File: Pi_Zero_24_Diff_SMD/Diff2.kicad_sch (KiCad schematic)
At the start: 14 parts, among them J7 Diff Out, J8 Diff Out, U7 AM26C31, U8 AM26C31

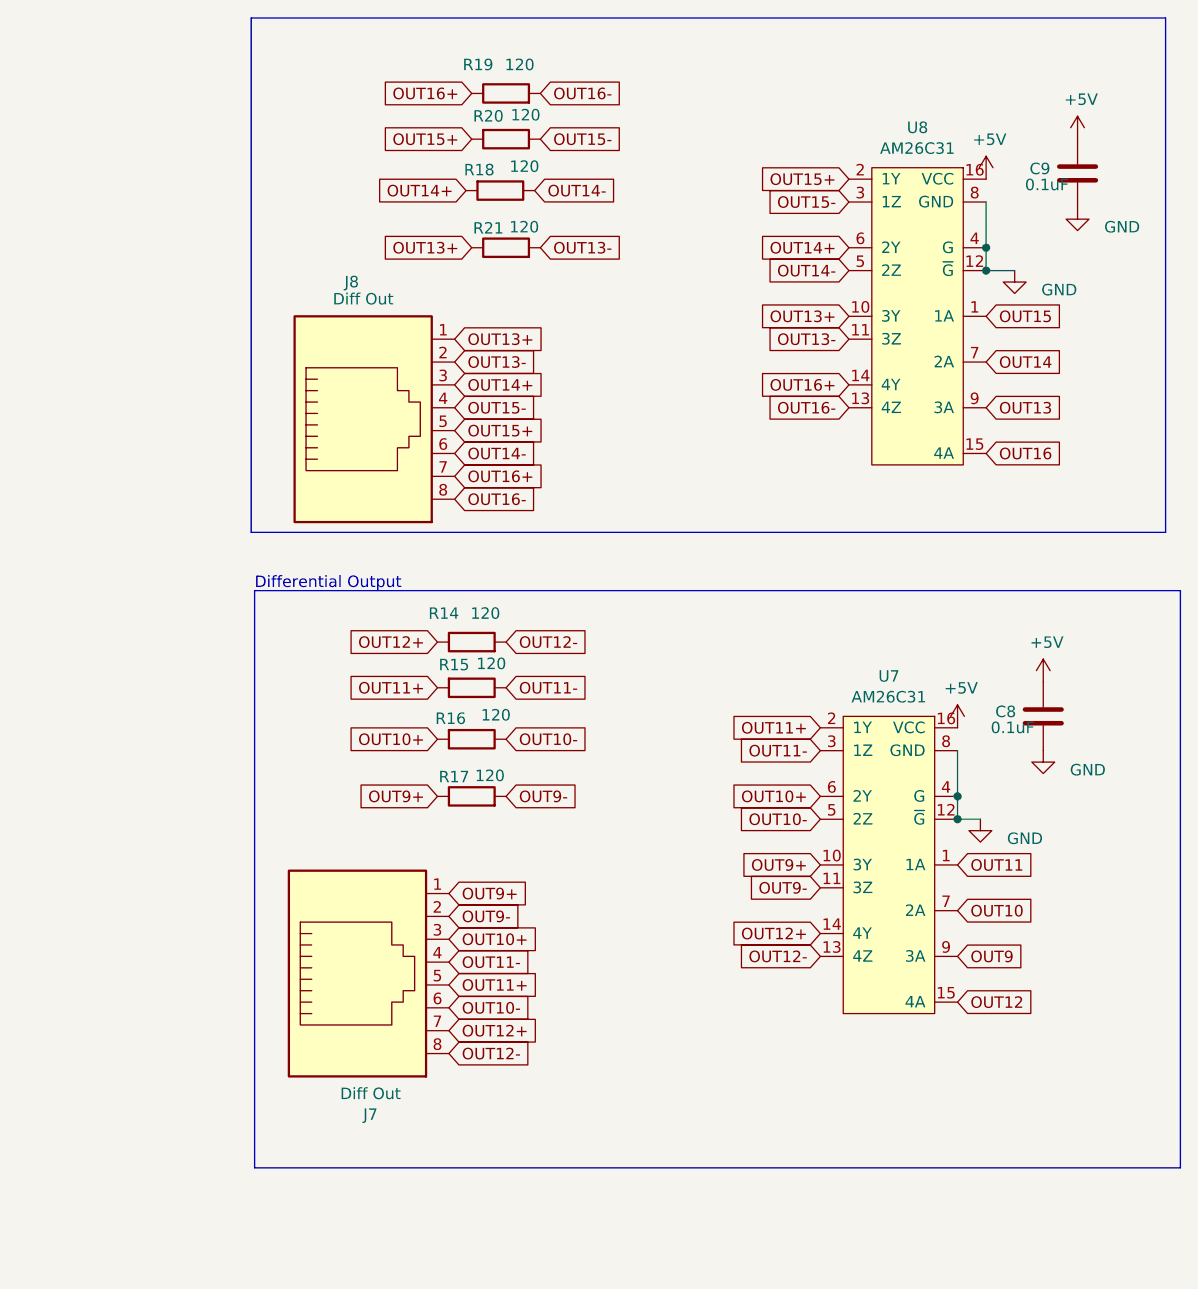
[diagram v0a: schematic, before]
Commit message: working on routing
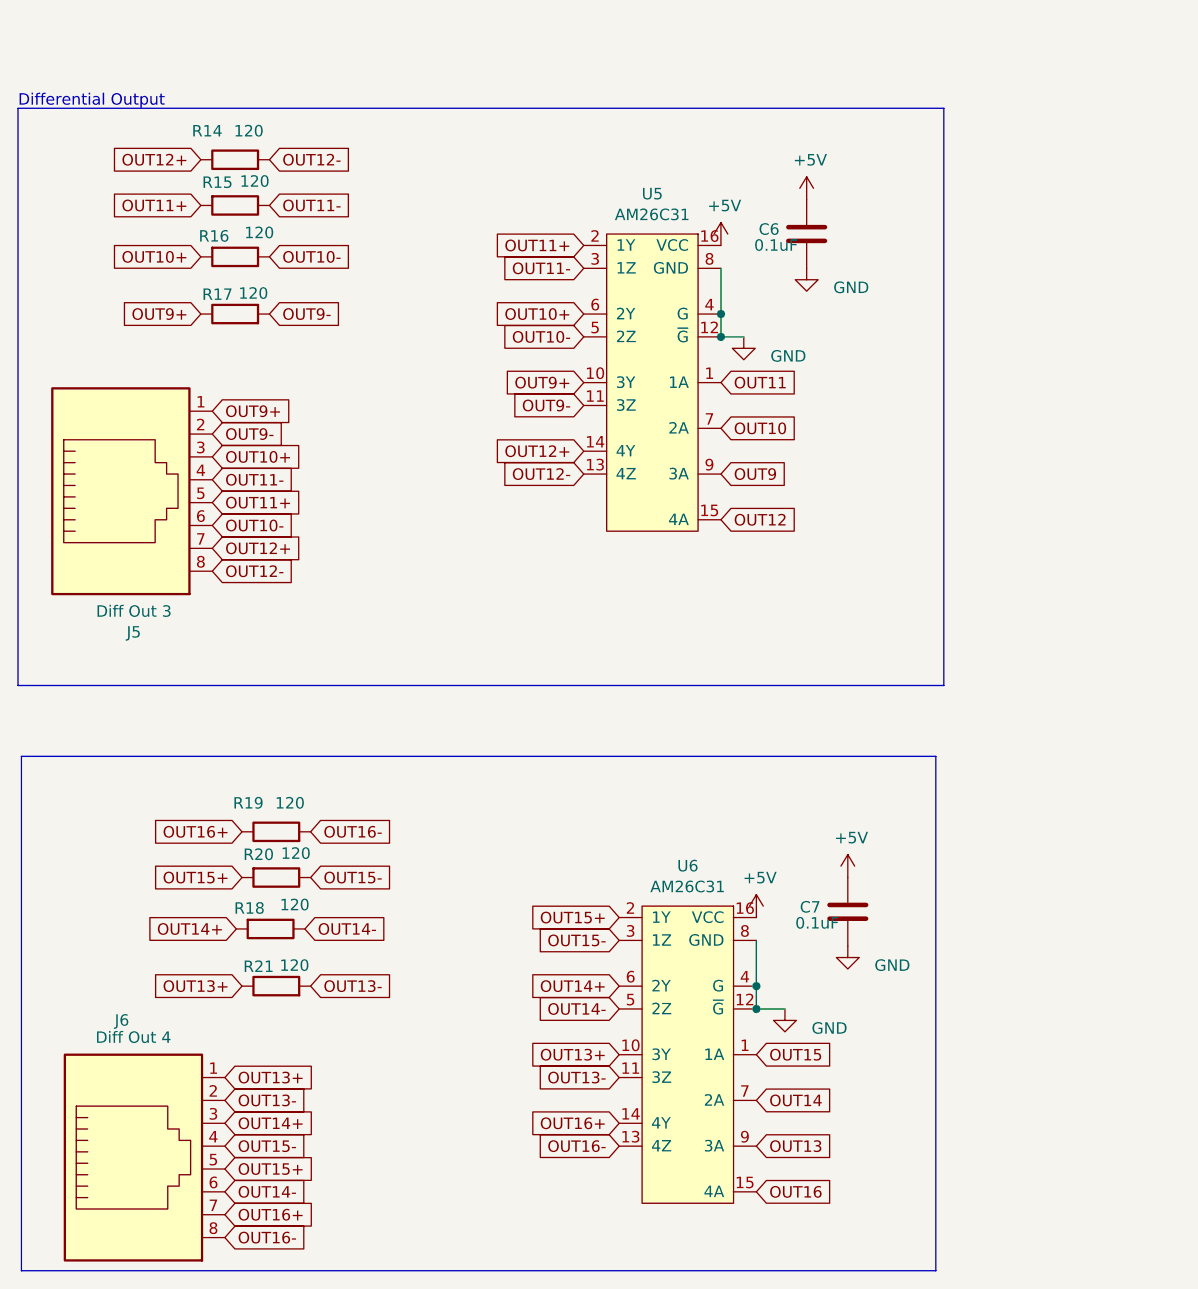
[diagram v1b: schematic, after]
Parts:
- J5: renamed from J7; value Diff Out -> Diff Out 3
- J6: renamed from J8; value Diff Out -> Diff Out 4
- renumbered C8 to C6, C9 to C7, U7 to U5, U8 to U6
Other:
- moved on the sheet: C6, C7, J5, J6, R14, R15, R16, R17, R18, R19, R20, R21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
